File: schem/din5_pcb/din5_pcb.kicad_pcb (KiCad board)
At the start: 2 copper layers, 62 parts, among them J1 Conn_01x03_Male, J101 DIN-5_180degree, J102 DIN-5_180degree, J103 DIN-5_180degree, J104 DIN-5_180degree, J2 2x3 female, J201 DIN-5_180degree, J202 DIN-5_180degree, J203 DIN-5_180degree, J204 DIN-5_180degree, J3 2x3 female, U1 74HCT245, U101 HCPL-2630, U102 HCPL-2630, U2 74HC595, U3 74HC165

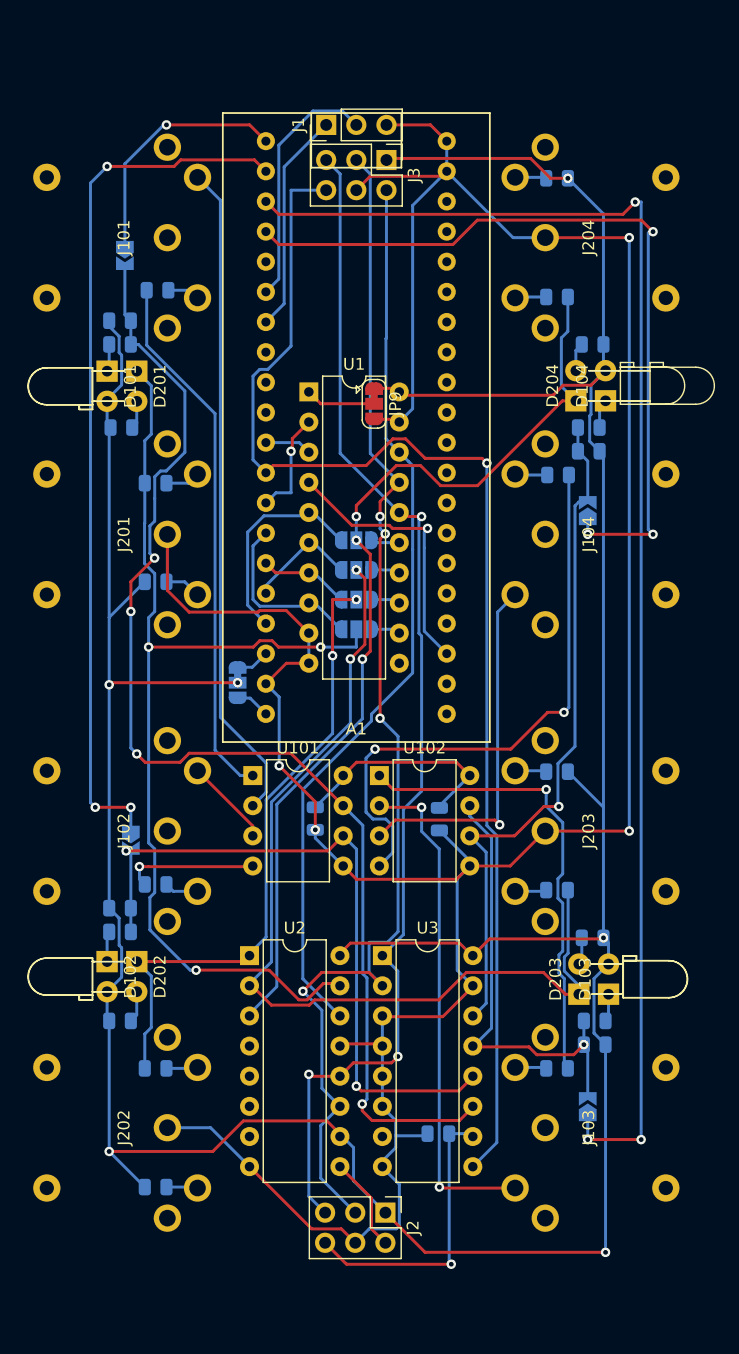
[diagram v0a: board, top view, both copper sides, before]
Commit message: Re-order parts on din5_pcb
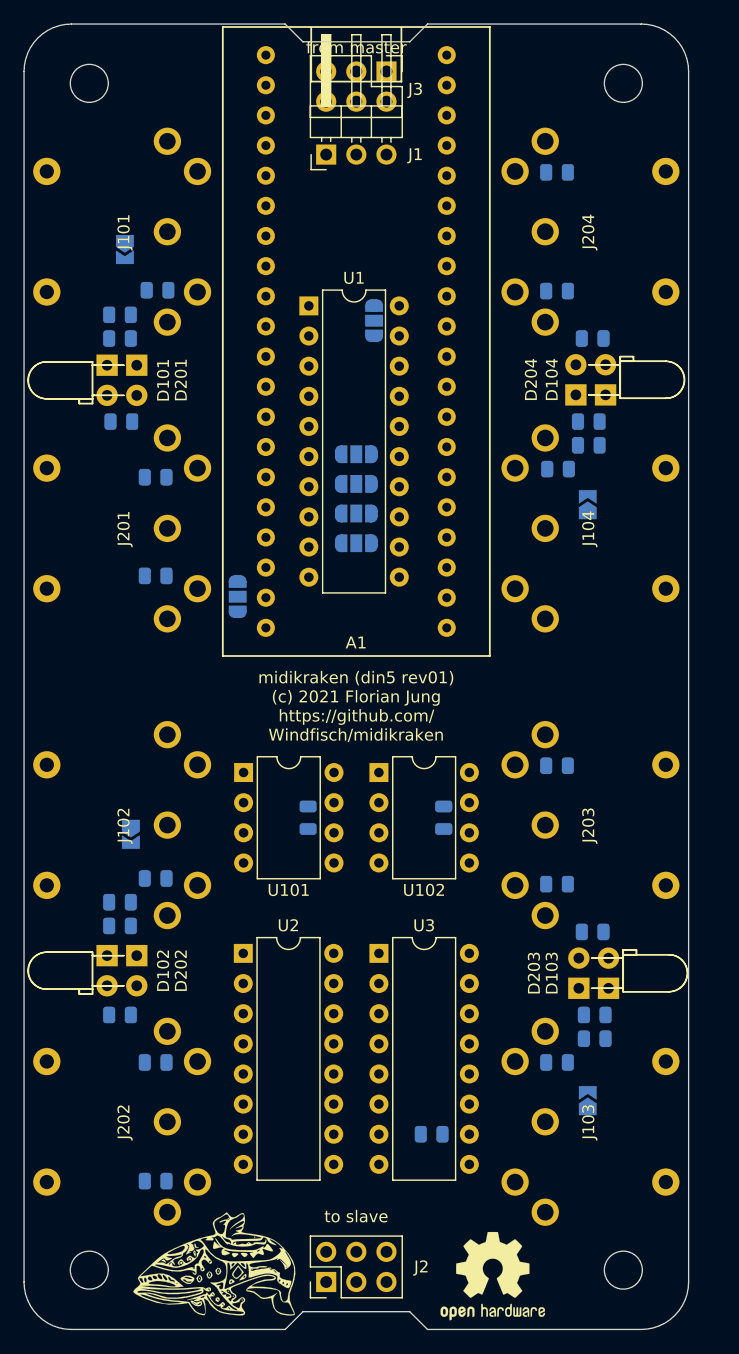
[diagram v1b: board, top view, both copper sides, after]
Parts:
- added G***: LOGO, windfisch:windfisch_smaller, F.Cu at (30.0, 109.5)
- added REF**: OSHW-Logo2_9.8x8mm_SilkScreen, Symbol:OSHW-Logo2_9.8x8mm_SilkScreen, F.Cu at (53.5, 110.5)
- added REF**: MountingHole_3.2mm_M3_DIN965, MountingHole:MountingHole_3.2mm_M3_DIN965, F.Cu at (64.5, 110.0)
- added REF**: MountingHole_3.2mm_M3_DIN965, MountingHole:MountingHole_3.2mm_M3_DIN965, F.Cu at (19.5, 110.0)
- added REF**: MountingHole_3.2mm_M3_DIN965, MountingHole:MountingHole_3.2mm_M3_DIN965, F.Cu at (64.5, 10.0)
- added REF**: MountingHole_3.2mm_M3_DIN965, MountingHole:MountingHole_3.2mm_M3_DIN965, F.Cu at (19.5, 10.0)
- A1: footprint footprints:BLUEPILL -> footprints:BLUEPILL-blackpill
- D104: footprint LED_THT:LED_D3.0mm_Horizontal_O3.81mm_Z6.0mm -> LED_THT:LED_D3.0mm_Horizontal_O1.27mm_Z2.0mm
- J1: footprint Connector_PinHeader_2.54mm:PinHeader_1x03_P2.54mm_Vertical -> Connector_PinHeader_2.54mm:PinHeader_1x03_P2.54mm_Horizontal
- JP14: footprint Jumper:SolderJumper-3_P1.3mm_Bridged12_RoundedPad1.0x1.5mm -> Jumper:SolderJumper-3_P1.3mm_Open_RoundedPad1.0x1.5mm
- JP9: footprint Jumper:SolderJumper-3_P1.3mm_Bridged12_RoundedPad1.0x1.5mm -> Jumper:SolderJumper-3_P1.3mm_Open_RoundedPad1.0x1.5mm; moved to B.Cu
- moved J2 7.68 mm to (39.5, 111.0), turned to 90 degrees
- moved J3 7.46 mm to (44.5, 9.00)
- moved A1 7.25 mm to (42.0, 31.8)
- moved JP14 7.25 mm to (32.0, 53.2)
- moved JP5 7.25 mm to (42.0, 48.8)
- moved JP6 7.25 mm to (42.0, 46.2)
- moved JP7 7.25 mm to (42.0, 43.8)
- moved JP8 7.25 mm to (42.0, 41.2)
- moved U1 7.25 mm to (38.0, 28.8)
- moved JP9 7.00 mm to (43.5, 30.0)
- moved J1 2.50 mm to (39.5, 16.0)
- moved U101 0.82 mm to (32.5, 68.1)
- moved C101 0.61 mm to (37.9, 71.9)
- moved R1 0.56 mm to (48.4, 98.5)
- moved U2 0.56 mm to (32.5, 83.3)
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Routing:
- net VCC: track 318.1 -> 0.00 mm, vias 6 -> 0
- net GND: track 252.1 -> 0.00 mm, vias 4 -> 0
- net Net-(A1-PadPB14): track 118.0 -> 0.00 mm, vias 3 -> 0
- net MISO_MIDI: track 110.1 -> 0.00 mm, vias 1 -> 0
- net SCK_MIDI_5: track 104.7 -> 0.00 mm, vias 4 -> 0
- net in0: track 103.1 -> 0.00 mm, vias 4 -> 0
- net STROBE_MIDI_5: track 102.3 -> 0.00 mm, vias 3 -> 0
- net out0: track 87.3 -> 0.00 mm, vias 3 -> 0
- net out3: track 80.6 -> 0.00 mm, vias 3 -> 0
- net out2: track 79.0 -> 0.00 mm, vias 2 -> 0
- net MOSI_MIDI_5: track 75.7 -> 0.00 mm
- net Net-(A1-PadPB13): track 73.8 -> 0.00 mm, vias 3 -> 0
- net Net-(A1-PadPB15): track 67.1 -> 0.00 mm, vias 3 -> 0
- net in3: track 58.6 -> 0.00 mm, vias 1 -> 0
- net in1: track 57.9 -> 0.00 mm, vias 2 -> 0
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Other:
- board outline added: 56 x 110 mm
- board text added: "245"
- board text added: "3.3V"
- board text added: "541"
- board text added: "5V"
- board text added: "from master"
- board text added: "midikraken (din5 rev01) (c) 2021 Florian Jung https://github.com/ Windfisch/midikraken"
- board text added: "pass thru"
- board text added: "to slave"

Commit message: intermediate commit
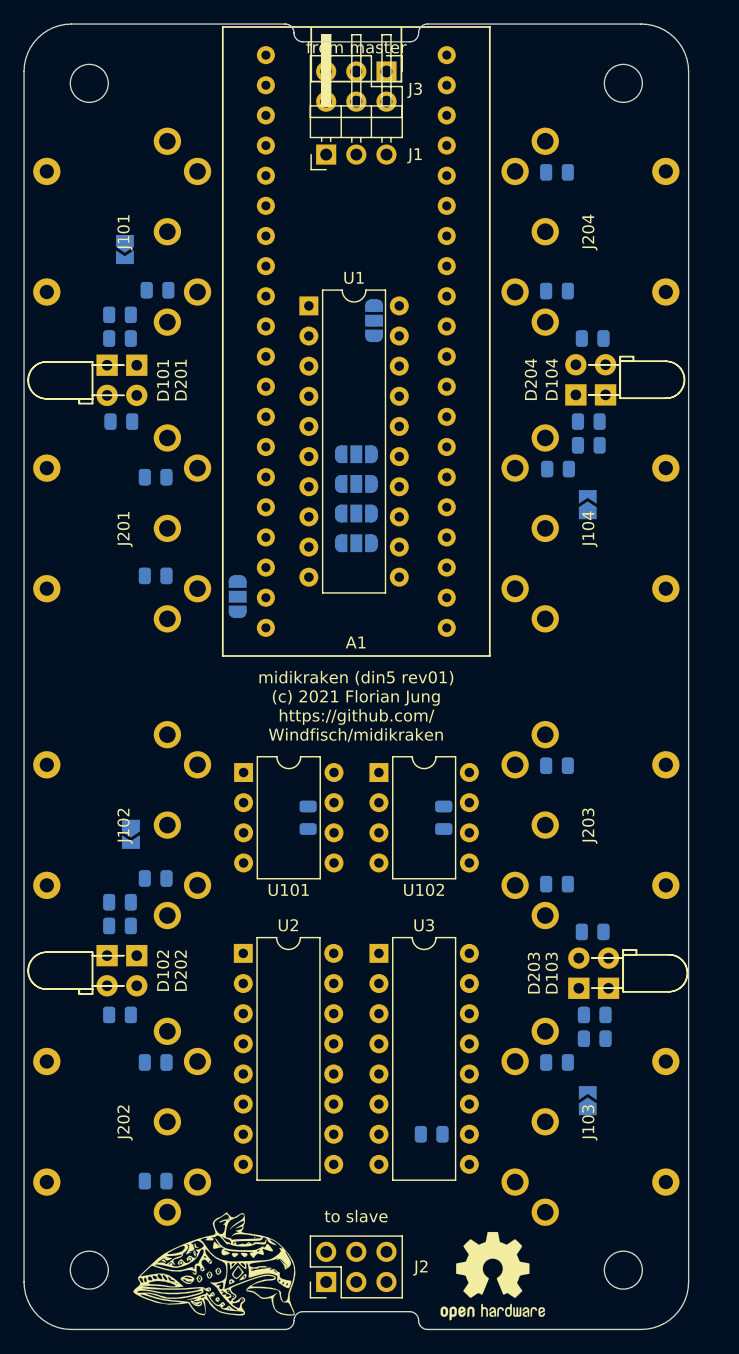
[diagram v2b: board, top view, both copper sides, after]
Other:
- outline, holes or cut-outs redrawn
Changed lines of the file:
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@@
   (general
     (thickness 1.6)
-    (drawings 28)
+    (drawings 32)
     (tracks 0)
     (zones 0)
@@
     )
   )
+  (gr_arc (start 46.5 5.75) (end 46.5 6.5) (angle -90) (layer Edge.Cuts) (width 0.05))
+  (gr_arc (start 48 5.75) (end 48 5) (angle -90) (layer Edge.Cuts) (width 0.05))
+  (gr_arc (start 37.5 5.75) (end 36.75 5.75) (angle -90) (layer Edge.Cuts) (width 0.05))
+  (gr_arc (start 36 5.75) (end 36.75 5.75) (angle -90) (layer Edge.Cuts) (width 0.05))
+  (gr_arc (start 46.5 114.25) (end 47.25 114.25) (angle -90) (layer Edge.Cuts) (width 0.05))
+  (gr_arc (start 48 114.25) (end 47.25 114.25) (angle -90) (layer Edge.Cuts) (width 0.05))
+  (gr_arc (start 37.5 114.25) (end 37.5 113.5) (angle -90) (layer Edge.Cuts) (width 0.05))
+  (gr_arc (start 36 114.25) (end 36 115) (angle -90) (layer Edge.Cuts) (width 0.05))
   (gr_line (start 14 9) (end 14 111) (layer Edge.Cuts) (width 0.05))
   (gr_line (start 36 5) (end 18 5) (layer Edge.Cuts) (width 0.05))
@@
   (gr_arc (start 18 111) (end 14 111) (angle -90) (layer Edge.Cuts) (width 0.05))
   (gr_arc (start 66 111) (end 66 115) (angle -90) (layer Edge.Cuts) (width 0.05))
-  (gr_line (start 46.5 113.5) (end 48 115) (layer Edge.Cuts) (width 0.05))
   (gr_line (start 37.5 113.5) (end 46.5 113.5) (layer Edge.Cuts) (width 0.05))
-  (gr_line (start 36 115) (end 37.5 113.5) (layer Edge.Cuts) (width 0.05))
-  (gr_line (start 46.5 6.5) (end 48 5) (layer Edge.Cuts) (width 0.05))
   (gr_line (start 37.5 6.5) (end 46.5 6.5) (layer Edge.Cuts) (width 0.05))
-  (gr_line (start 36 5) (end 37.5 6.5) (layer Edge.Cuts) (width 0.05))
   (gr_text "midikraken (din5 rev01)\n(c) 2021 Florian Jung\nhttps://github.com/\nWindfisch/midikraken" (at 42 62.5) (layer F.SilkS)
     (effects (font (size 1 1) (thickness 0.15)))
